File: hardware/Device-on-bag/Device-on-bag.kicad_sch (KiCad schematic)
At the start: 3 parts

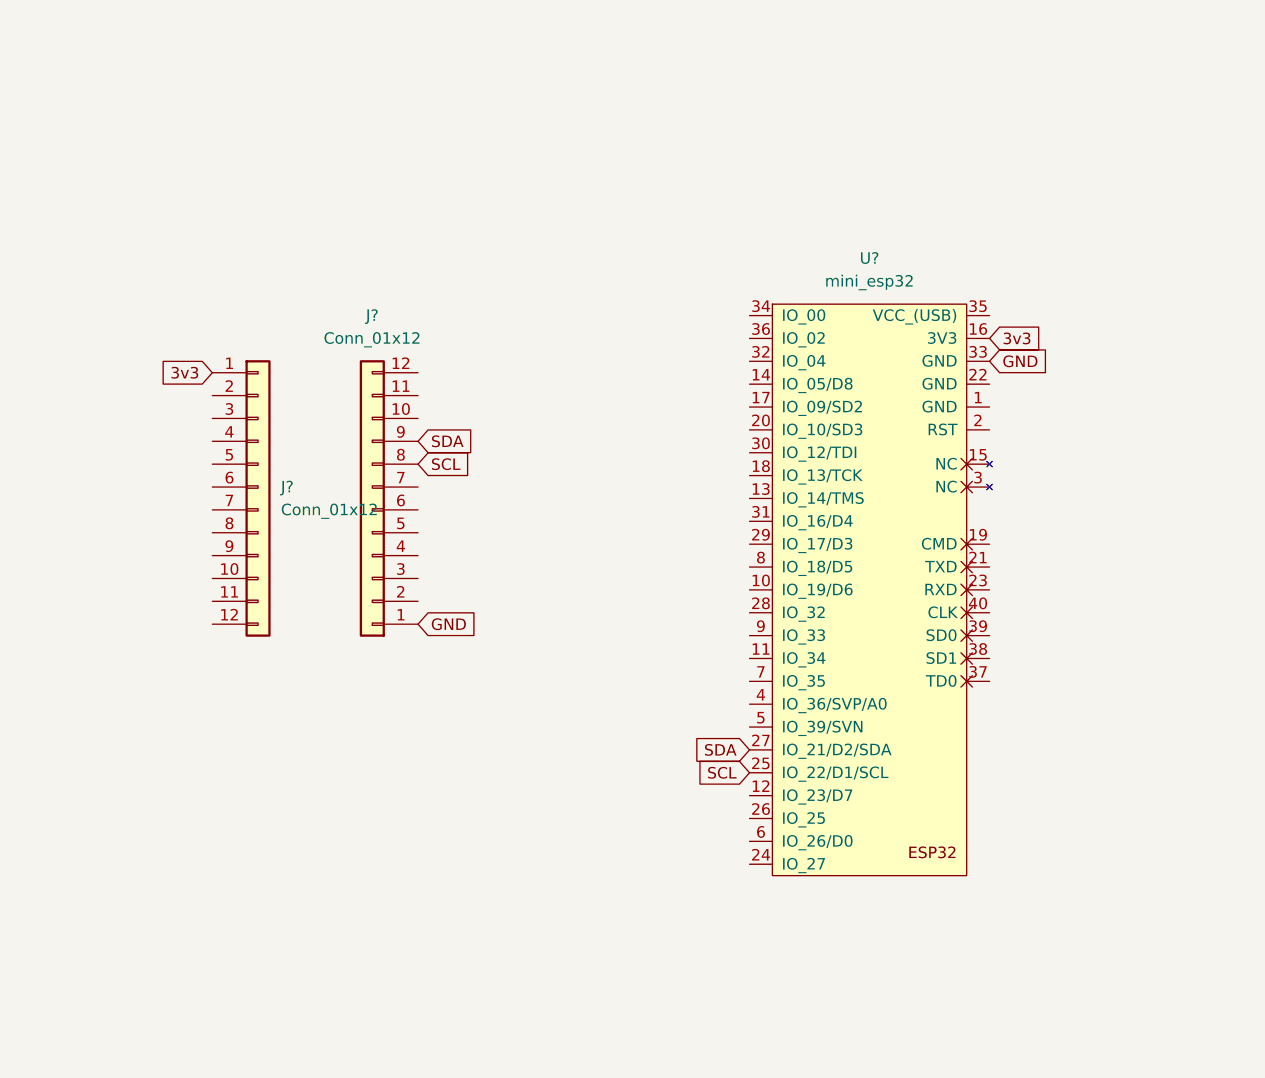
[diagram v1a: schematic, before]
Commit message: update
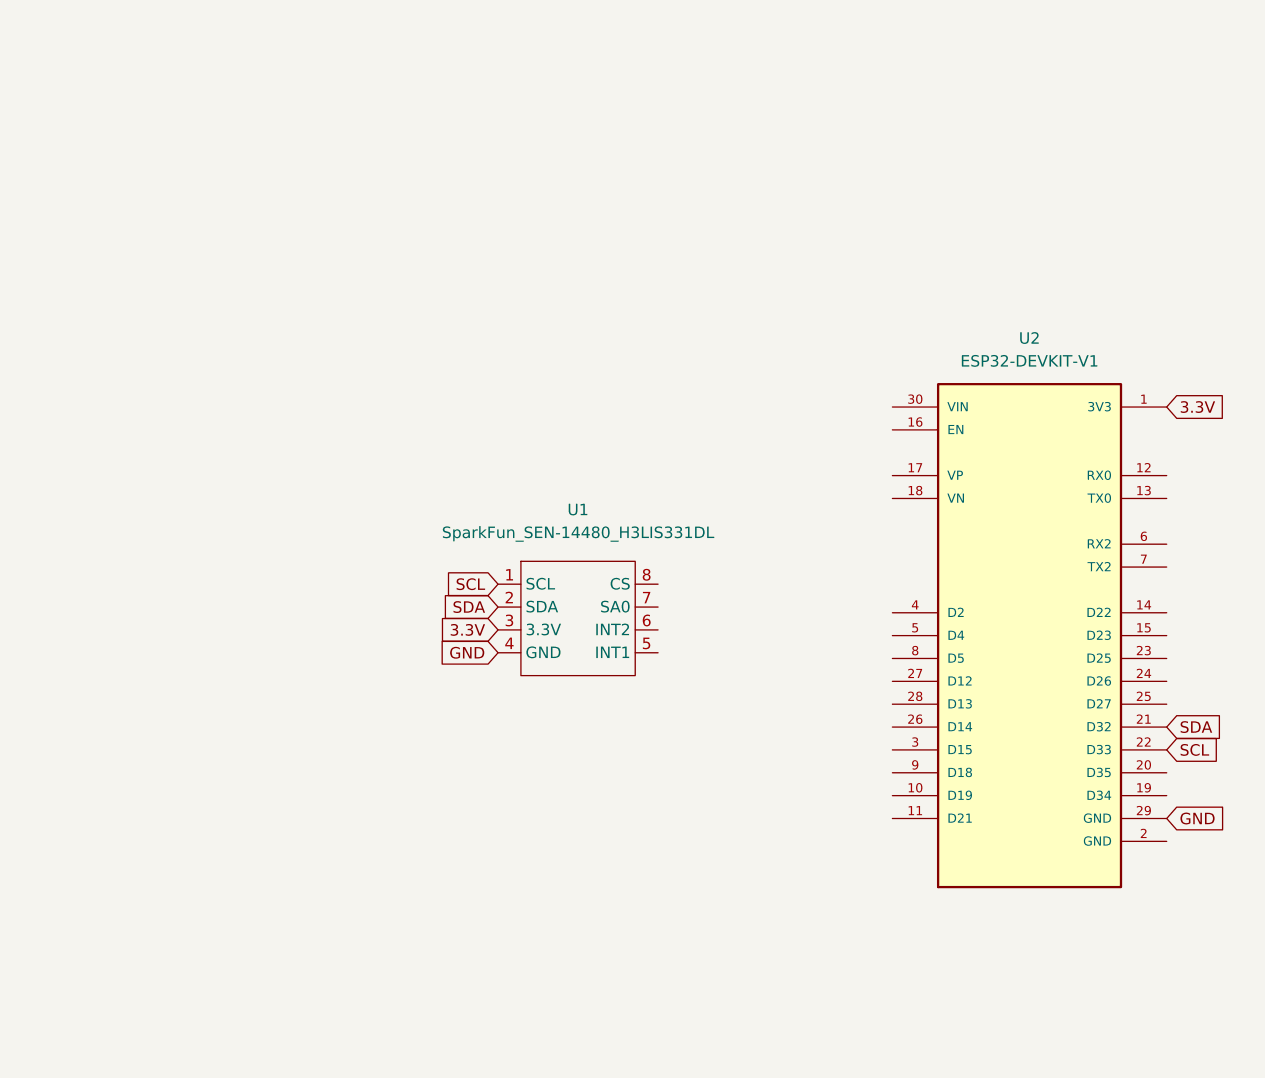
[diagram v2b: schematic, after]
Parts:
- removed J? (x2): Conn_01x12, Connector_PinSocket_2.54mm:PinSocket_1x11_P2.54mm_Vertical, symbol Connector_Generic:Conn_01x12
- removed U?: mini_esp32, ESP32_mini:ESP32_mini, symbol ESP32_mini:mini_esp32
- added U1: SparkFun_SEN-14480_H3LIS331DL, SparkFun_Tri_Axis_Accel_Breakout-H3LIS331DL:SparkFun_Tri_Axis_Accel_Breakout-H3LIS331DL, symbol H3LIS331DL:SparkFun_SEN-14480_H3LIS331DL
- added U2: ESP32-DEVKIT-V1, MODULE_ESP32_DEVKIT_V1, symbol ESP32-DEVKIT-V1:ESP32-DEVKIT-V1
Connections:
- net GND: now also U1.4 (GND), U2.29 (GND)
- net SCL: now also U1.1 (SCL), U2.22 (D33)
- net SDA: now also U1.2 (SDA), U2.21 (D32)
- new net 3.3V: U1.3 (3.3V), U2.1 (3V3)
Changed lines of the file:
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@@
 (kicad_sch (version 20211123) (generator eeschema)
   (paper "A4")
-  (global_label "3v3" (shape input) (at 86.36 69.85 180) (fields_autoplaced)
+  (global_label "3.3V" (shape input) (at 118.11 98.425 180) (fields_autoplaced)
     (effects (font (size 1.27 1.27)) (justify right))
-    (property "Intersheet References" "${INTERSHEET_REFS}" (id 0) (at 80.5602 69.9294 0)
+    (property "Intersheet References" "${INTERSHEET_REFS}" (id 0) (at 111.5845 98.5044 0)
       (effects (font (size 1.27 1.27)) (justify right) hide)
     )
   )
-  (global_label "SCL" (shape input) (at 146.05 114.3 180) (fields_autoplaced)
+  (global_label "SCL" (shape input) (at 192.405 111.76 0) (fields_autoplaced)
+    (effects (font (size 1.27 1.27)) (justify left))
+    (property "Intersheet References" "${INTERSHEET_REFS}" (id 0) (at 198.3257 111.6806 0)
+      (effects (font (size 1.27 1.27)) (justify left) hide)
+    )
+  )
+  (global_label "GND" (shape input) (at 118.11 100.965 180) (fields_autoplaced)
     (effects (font (size 1.27 1.27)) (justify right))
-    (property "Intersheet References" "${INTERSHEET_REFS}" (id 0) (at 140.1293 114.3794 0)
+    (property "Intersheet References" "${INTERSHEET_REFS}" (id 0) (at 111.8264 100.8856 0)
       (effects (font (size 1.27 1.27)) (justify right) hide)
     )
   )
-  (global_label "GND" (shape input) (at 172.72 68.58 0) (fields_autoplaced)
+  (global_label "GND" (shape input) (at 192.405 119.38 0) (fields_autoplaced)
     (effects (font (size 1.27 1.27)) (justify left))
-    (property "Intersheet References" "${INTERSHEET_REFS}" (id 0) (at 179.0036 68.5006 0)
+    (property "Intersheet References" "${INTERSHEET_REFS}" (id 0) (at 198.6886 119.4594 0)
       (effects (font (size 1.27 1.27)) (justify left) hide)
     )
   )
-  (global_label "SCL" (shape input) (at 109.22 80.01 0) (fields_autoplaced)
+  (global_label "3.3V" (shape input) (at 192.405 73.66 0) (fields_autoplaced)
     (effects (font (size 1.27 1.27)) (justify left))
-    (property "Intersheet References" "${INTERSHEET_REFS}" (id 0) (at 115.1407 79.9306 0)
+    (property "Intersheet References" "${INTERSHEET_REFS}" (id 0) (at 198.9305 73.5806 0)
       (effects (font (size 1.27 1.27)) (justify left) hide)
     )
   )
-  (global_label "SDA" (shape input) (at 146.05 111.76 180) (fields_autoplaced)
+  (global_label "SDA" (shape input) (at 192.405 109.22 0) (fields_autoplaced)
+    (effects (font (size 1.27 1.27)) (justify left))
+    (property "Intersheet References" "${INTERSHEET_REFS}" (id 0) (at 198.3862 109.1406 0)
+      (effects (font (size 1.27 1.27)) (justify left) hide)
+    )
+  )
+  (global_label "SCL" (shape input) (at 118.11 93.345 180) (fields_autoplaced)
     (effects (font (size 1.27 1.27)) (justify right))
-    (property "Intersheet References" "${INTERSHEET_REFS}" (id 0) (at 140.0688 111.8394 0)
+    (property "Intersheet References" "${INTERSHEET_REFS}" (id 0) (at 112.1893 93.4244 0)
       (effects (font (size 1.27 1.27)) (justify right) hide)
     )
   )
-  (global_label "GND" (shape input) (at 109.22 97.79 0) (fields_autoplaced)
-    (effects (font (size 1.27 1.27)) (justify left))
-    (property "Intersheet References" "${INTERSHEET_REFS}" (id 0) (at 115.5036 97.7106 0)
-      (effects (font (size 1.27 1.27)) (justify left) hide)
+  (global_label "SDA" (shape input) (at 118.11 95.885 180) (fields_autoplaced)
+    (effects (font (size 1.27 1.27)) (justify right))
+    (property "Intersheet References" "${INTERSHEET_REFS}" (id 0) (at 112.1288 95.9644 0)
+      (effects (font (size 1.27 1.27)) (justify right) hide)
     )
   )
-  (global_label "3v3" (shape input) (at 172.72 66.04 0) (fields_autoplaced)
-    (effects (font (size 1.27 1.27)) (justify left))
-    (property "Intersheet References" "${INTERSHEET_REFS}" (id 0) (at 178.5198 65.9606 0)
-      (effects (font (size 1.27 1.27)) (justify left) hide)
-    )
-  )
-  (global_label "SDA" (shape input) (at 109.22 77.47 0) (fields_autoplaced)
-    (effects (font (size 1.27 1.27)) (justify left))
-    (property "Intersheet References" "${INTERSHEET_REFS}" (id 0) (at 115.2012 77.3906 0)
-      (effects (font (size 1.27 1.27)) (justify left) hide)
-    )
-  )
-  (symbol (lib_id "ESP32_mini:mini_esp32") (at 158.75 60.96 0) (unit 1)
+  (symbol (lib_id "H3LIS331DL:SparkFun_SEN-14480_H3LIS331DL") (at 127 97.155 0) (unit 1)
     (in_bom yes) (on_board yes) (fields_autoplaced)
-    (property "Reference" "U?" (id 0) (at 159.385 57.15 0))
-    (property "Value" "mini_esp32" (id 1) (at 159.385 59.69 0))
-    (property "Footprint" "ESP32_mini:ESP32_mini" (id 2) (at 162.56 58.42 0)
+    (property "Reference" "U1" (id 0) (at 127 85.09 0))
+    (property "Value" "SparkFun_SEN-14480_H3LIS331DL" (id 1) (at 127 87.63 0))
+    (property "Footprint" "SparkFun_Tri_Axis_Accel_Breakout-H3LIS331DL:SparkFun_Tri_Axis_Accel_Breakout-H3LIS331DL" (id 2) (at 127 97.155 0)
       (effects (font (size 1.27 1.27)) hide)
     )
-    (property "Datasheet" "" (id 3) (at 162.56 58.42 0)
+    (property "Datasheet" "" (id 3) (at 127 97.155 0)
       (effects (font (size 1.27 1.27)) hide)
     )
@@
     (pin "4")
     (pin "5")
+    (pin "6")
+    (pin "7")
+    (pin "8")
+  )
+  (symbol (lib_id "ESP32-DEVKIT-V1:ESP32-DEVKIT-V1") (at 177.165 99.06 0) (unit 1)
+    (in_bom yes) (on_board yes) (fields_autoplaced)
+    (property "Reference" "U2" (id 0) (at 177.165 66.04 0))
+    (property "Value" "ESP32-DEVKIT-V1" (id 1) (at 177.165 68.58 0))
+    (property "Footprint" "MODULE_ESP32_DEVKIT_V1" (id 2) (at 165.735 62.23 0)
+      (effects (font (size 1.27 1.27)) (justify left bottom) hide)
+    )
+    (property "Datasheet" "" (id 3) (at 177.165 99.06 0)
+      (effects (font (size 1.27 1.27)) (justify left bottom) hide)
+    )
+    (property "STANDARD" "Manufacturer Recommendations" (id 4) (at 163.195 64.77 0)
+      (effects (font (size 1.27 1.27)) (justify left bottom) hide)
+    )
+    (property "PARTREV" "N/A" (id 5) (at 184.785 67.31 0)
+      (effects (font (size 1.27 1.27)) (justify left bottom) hide)
+    )
+    (property "MANUFACTURER" "DOIT" (id 6) (at 191.135 62.23 0)
+      (effects (font (size 1.27 1.27)) (justify left bottom) hide)
+    )
+    (property "MAXIMUM_PACKAGE_HEIGHT" "6.8 mm" (id 7) (at 183.515 69.85 0)
+      (effects (font (size 1.27 1.27)) (justify left bottom) hide)
+    )
+    (pin "1")
     (pin "10")
     (pin "11")
@@
     (pin "18")
     (pin "19")
+    (pin "2")
     (pin "20")
     (pin "21")
@@
     (pin "28")
     (pin "29")
+    (pin "3")
     (pin "30")
-    (pin "31")
-    (pin "32")
-    (pin "33")
-    (pin "34")
-    (pin "35")
-    (pin "36")
-    (pin "37")
-    (pin "38")
-    (pin "39")
-    (pin "40")
-    (pin "6")
-    (pin "7")
-    (pin "8")
-    (pin "9")
-  )
-  (symbol (lib_id "Connector_Generic:Conn_01x12") (at 91.44 82.55 0) (unit 1)
-    (in_bom yes) (on_board yes) (fields_autoplaced)
-    (property "Reference" "J?" (id 0) (at 93.98 82.5499 0)
-      (effects (font (size 1.27 1.27)) (justify left))
-    )
-    (property "Value" "Conn_01x12" (id 1) (at 93.98 85.0899 0)
-      (effects (font (size 1.27 1.27)) (justify left))
-    )
-    (property "Footprint" "Connector_PinSocket_2.54mm:PinSocket_1x11_P2.54mm_Vertical" (id 2) (at 91.44 82.55 0)
-      (effects (font (size 1.27 1.27)) hide)
-    )
-    (property "Datasheet" "~" (id 3) (at 91.44 82.55 0)
-      (effects (font (size 1.27 1.27)) hide)
-    )
-    (pin "1")
-    (pin "10")
-    (pin "11")
-    (pin "12")
-    (pin "2")
-    (pin "3")
-    (pin "4")
-    (pin "5")
-    (pin "6")
-    (pin "7")
-    (pin "8")
-    (pin "9")
-  )
-  (symbol (lib_id "Connector_Generic:Conn_01x12") (at 104.14 85.09 180) (unit 1)
-    (in_bom yes) (on_board yes) (fields_autoplaced)
-    (property "Reference" "J?" (id 0) (at 104.14 63.5 0))
-    (property "Value" "Conn_01x12" (id 1) (at 104.14 66.04 0))
-    (property "Footprint" "Connector_PinSocket_2.54mm:PinSocket_1x11_P2.54mm_Vertical" (id 2) (at 104.14 85.09 0)
-      (effects (font (size 1.27 1.27)) hide)
-    )
-    (property "Datasheet" "~" (id 3) (at 104.14 85.09 0)
-      (effects (font (size 1.27 1.27)) hide)
-    )
-    (pin "1")
-    (pin "10")
-    (pin "11")
-    (pin "12")
-    (pin "2")
-    (pin "3")
     (pin "4")
     (pin "5")
@@
   )
   (symbol_instances
-    (path "/b65a8ad3-ec23-4ae3-b007-02d5070d82ec"
-      (reference "J?") (unit 1) (value "Conn_01x12") (footprint "Connector_PinSocket_2.54mm:PinSocket_1x11_P2.54mm_Vertical")
+    (path "/bdadbb5c-7221-4007-9a12-2ce8f2e20049"
+      (reference "U1") (unit 1) (value "SparkFun_SEN-14480_H3LIS331DL") (footprint "SparkFun_Tri_Axis_Accel_Breakout-H3LIS331DL:SparkFun_Tri_Axis_Accel_Breakout-H3LIS331DL")
     )
-    (path "/def40bea-bd6a-4bd4-85d6-38a0bc393684"
-      (reference "J?") (unit 1) (value "Conn_01x12") (footprint "Connector_PinSocket_2.54mm:PinSocket_1x11_P2.54mm_Vertical")
-    )
-    (path "/1f881f44-1f04-46f4-a465-f1747e7275b2"
-      (reference "U?") (unit 1) (value "mini_esp32") (footprint "ESP32_mini:ESP32_mini")
+    (path "/f3434164-7b41-4e11-b256-2613206fdd17"
+      (reference "U2") (unit 1) (value "ESP32-DEVKIT-V1") (footprint "MODULE_ESP32_DEVKIT_V1")
     )
   )
